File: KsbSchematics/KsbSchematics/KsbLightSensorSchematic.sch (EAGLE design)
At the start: 31 parts, among them IC1 7805L, IC2 LM311N, U1 ATTINY84

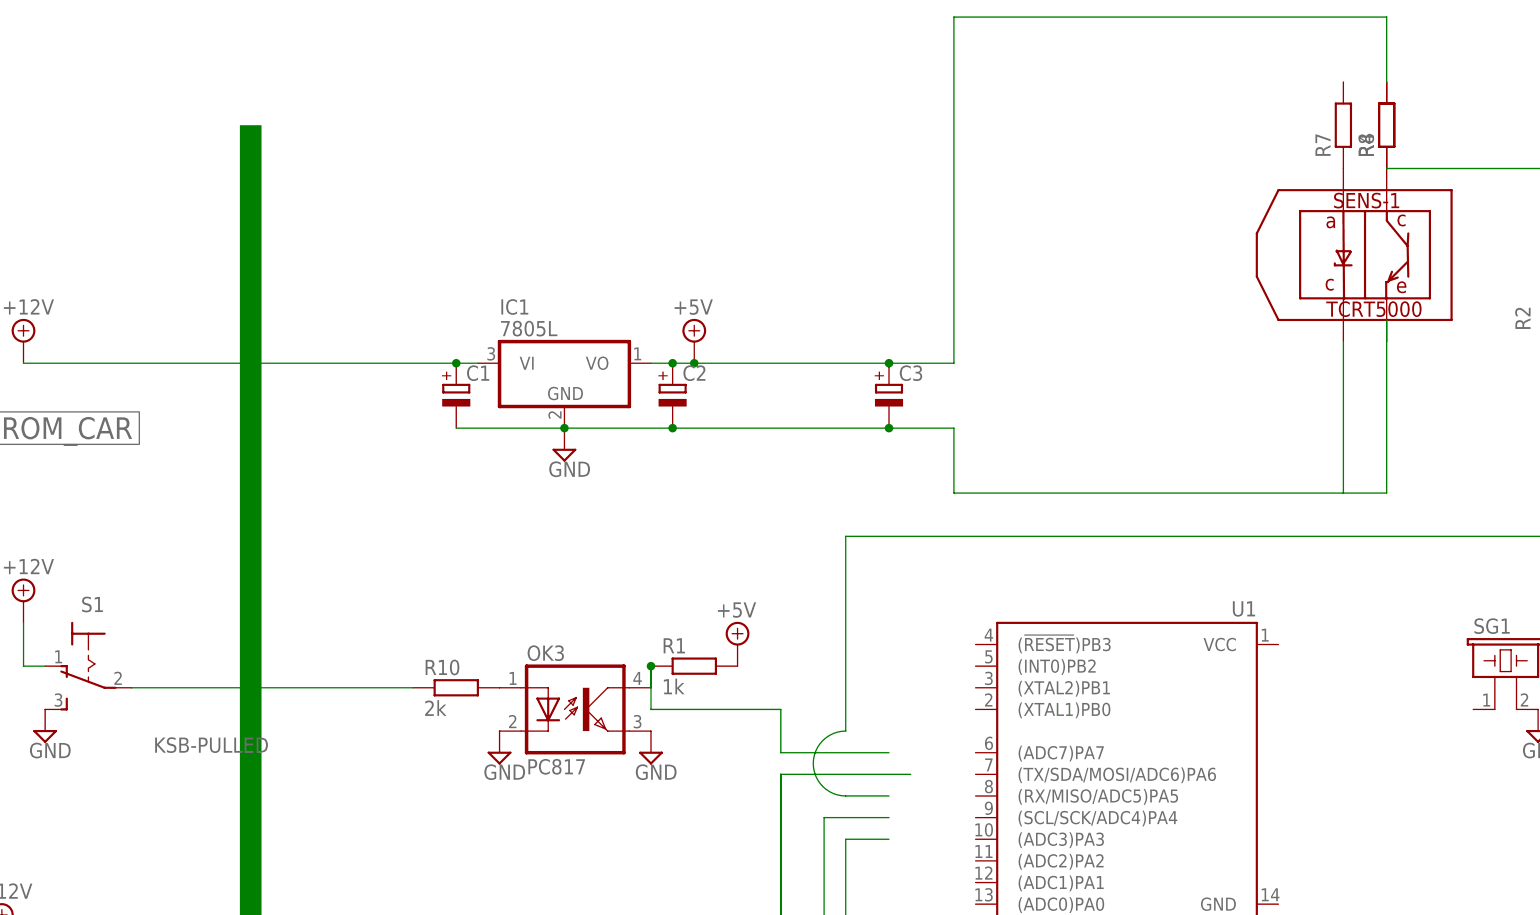
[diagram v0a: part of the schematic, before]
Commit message: schematics change
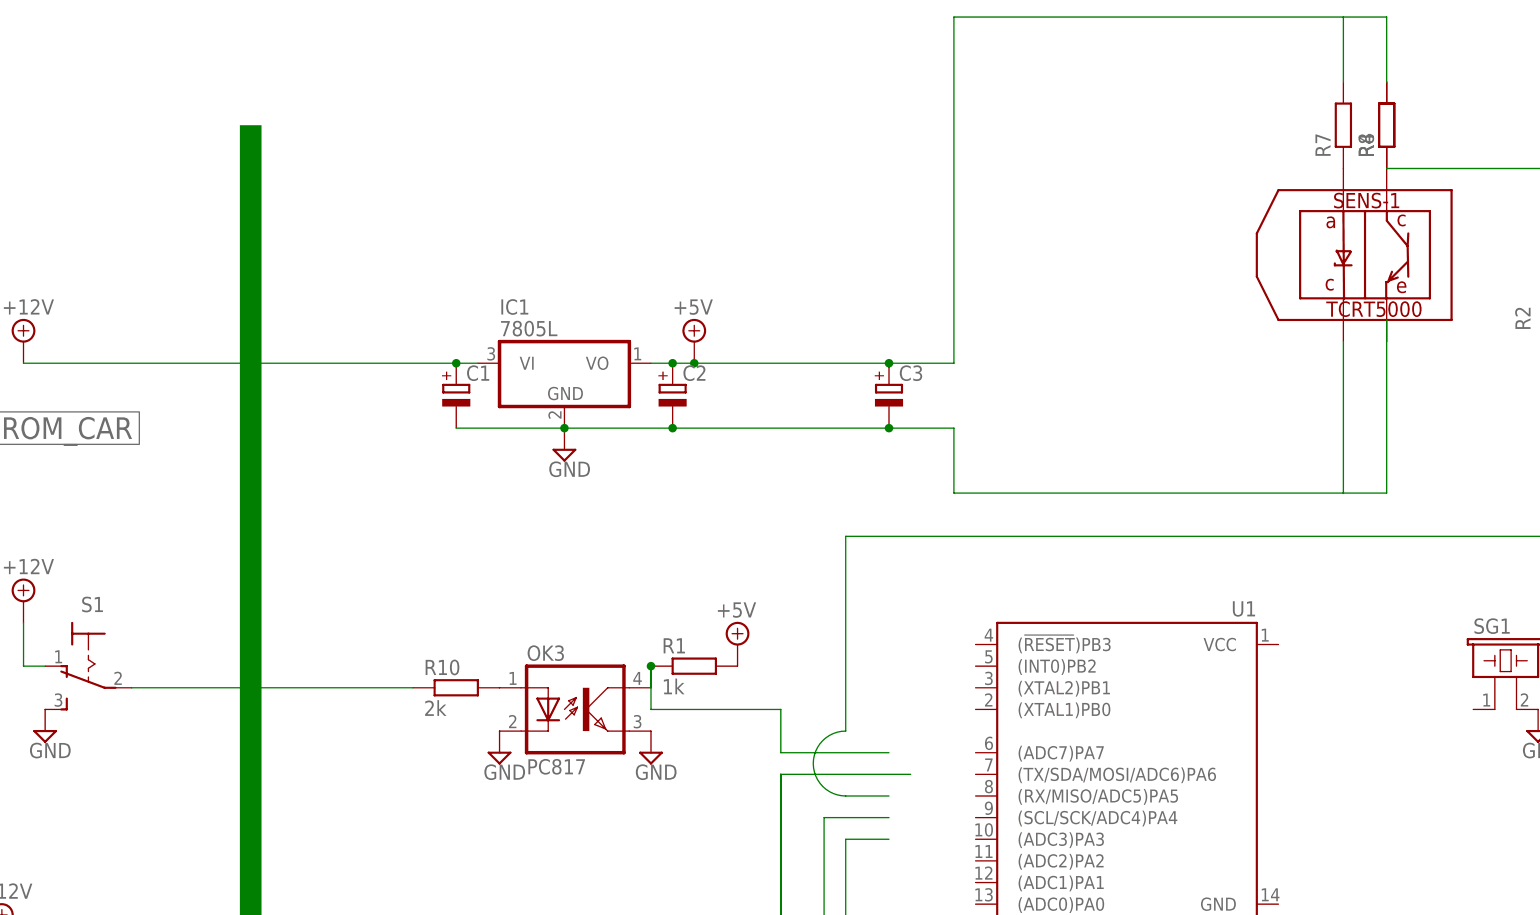
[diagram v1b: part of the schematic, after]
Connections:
- net +12V: now also R7.2
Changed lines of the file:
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@@
 <pinref part="C3" gate="G$1" pin="+"/>
 <wire x1="43.18" y1="124.46" x2="43.18" y2="165.1" width="0.1524" layer="91"/>
-<wire x1="43.18" y1="165.1" x2="93.98" y2="165.1" width="0.1524" layer="91"/>
+<wire x1="43.18" y1="165.1" x2="88.9" y2="165.1" width="0.1524" layer="91"/>
 <pinref part="R4" gate="G$1" pin="2"/>
 <pinref part="R8" gate="G$1" pin="2"/>
+<wire x1="88.9" y1="165.1" x2="93.98" y2="165.1" width="0.1524" layer="91"/>
 <wire x1="93.98" y1="165.1" x2="93.98" y2="157.48" width="0.1524" layer="91"/>
+<pinref part="R7" gate="G$1" pin="2"/>
+<wire x1="88.9" y1="165.1" x2="88.9" y2="157.48" width="0.1524" layer="91"/>
 </segment>
 <segment>
@@
 <pinref part="R10" gate="G$1" pin="1"/>
 <label x="-91.44" y="83.82" size="2.54" layer="95"/>
-<label x="-50.8" y="78.74" size="1.778" layer="95"/>
-</segment>
-</net>
+</segment>
+</net>
